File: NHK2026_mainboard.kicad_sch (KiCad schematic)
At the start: 2 parts, among them J1 ABS_Encoder, U1 STM32H753ZITx

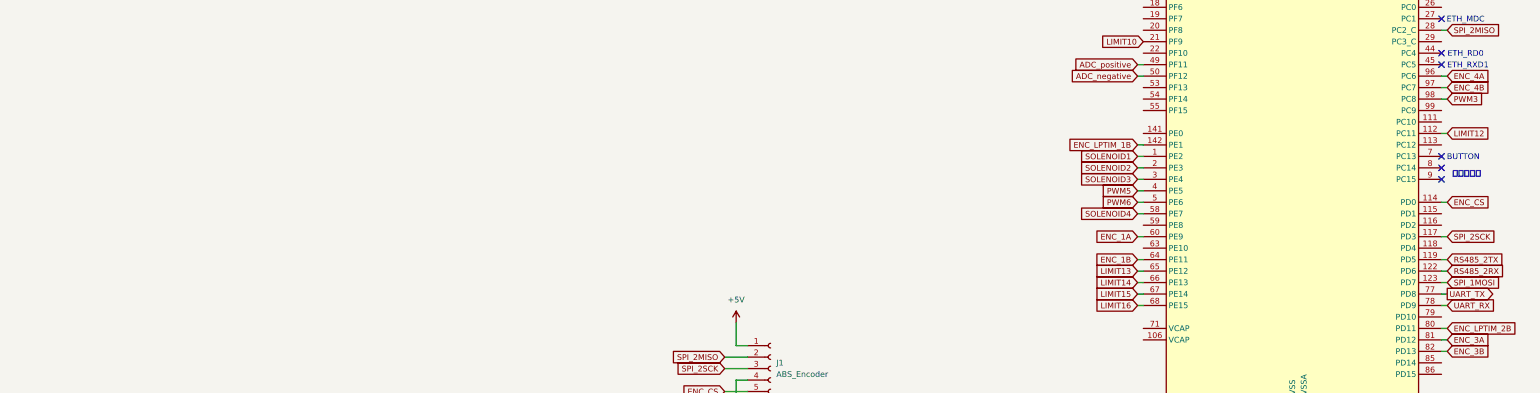
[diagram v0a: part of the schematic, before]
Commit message: 今日はここまで
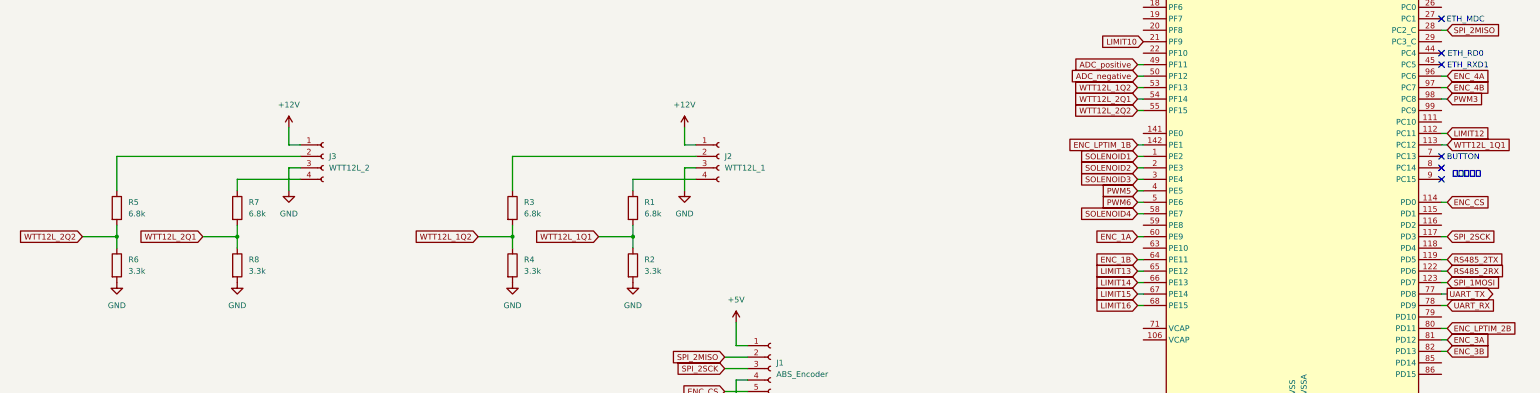
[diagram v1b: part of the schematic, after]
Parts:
- added J2: WTT12L_1, symbol Connector:Conn_01x04_Socket
- added J3: WTT12L_2, symbol Connector:Conn_01x04_Socket
- added R1, R3, R5, R7: 6.8k, symbol Device:R
- added R2, R4, R6, R8: 3.3k, symbol Device:R
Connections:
- net GND: now also J2.3 (Pin_3), J3.3 (Pin_3), R2.2, R4.2, R6.2, R8.2
- net WTT12L_1Q1: now reaches U1.113 (PC12)
- net WTT12L_1Q1: now also R1.2, R2.1
- net WTT12L_1Q2: now reaches U1.53 (PF13)
- net WTT12L_1Q2: now also R3.2, R4.1
- net WTT12L_2Q1: now reaches U1.54 (PF14)
- net WTT12L_2Q1: now also R7.2, R8.1
- net WTT12L_2Q2: now reaches U1.55 (PF15)
- net WTT12L_2Q2: now also R5.2, R6.1
- new net: J2.2 (Pin_2), R3.1
- new net: J3.2 (Pin_2), R5.1
- new net: J3.4 (Pin_4), R7.1
- new net: J2.4 (Pin_4), R1.1
- new net +12V: J2.1 (Pin_1), J3.1 (Pin_1)

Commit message: 恥を捨て豊橋スタイル丸パクリ
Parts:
- removed J2: WTT12L_1, symbol Connector:Conn_01x04_Socket
- removed J3: WTT12L_2, symbol Connector:Conn_01x04_Socket
- removed R1, R3, R5, R7: 6.8k, symbol Device:R
- removed R2, R4, R6, R8: 3.3k, symbol Device:R
- added C?: 0.1u, symbol Device:C
- added C?: 0.1u, Capacitor_SMD:C_0603_1608Metric_Pad1.08x0.95mm_HandSolder, symbol Device:C
- added J?: SPI, symbol Connector:Conn_01x04_Socket
- added J?: ADC, symbol Connector:Conn_01x02_Socket
- added J?: I2C, symbol Connector:Conn_01x03_Socket
- added J?: SOLENOID_1, Connector_JST:JST_XH_S5B-XH-A-1_1x05_P2.50mm_Horizontal, symbol Connector:Conn_01x05_Socket
- added U?: BNO055, MyLib:BNO055, symbol MyLib:BNO055
- added U?: TXRX_pokayoke, Mylib:TXRX_pokayoke, symbol MyLib:TXRX_pokayoke
- renumbered J1 to J?, U1 to U?
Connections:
- net +5V: now also C?.1
- net ADC_negative: now also J?.2 (Pin_2)
- net ADC_positive: now also J?.1 (Pin_1)
- net BNO_RX: now also U?.3 (RX1)
- net BNO_TX: now also U?.1 (TX1)
- net GND: now also C?.2, C?.2, J?.1 (Pin_1), J?.1 (Pin_1), J?.1 (Pin_1), U?.2 (GND), U?.6 (GND)
- net I2C_SCL: now also J?.3 (Pin_3)
- net I2C_SDA: now also J?.2 (Pin_2)
- net SOLENOID1: now also J?.2 (Pin_2)
- net SOLENOID2: now also J?.3 (Pin_3)
- net SOLENOID3: now also J?.4 (Pin_4)
- net SOLENOID4: now also J?.5 (Pin_5)
- net SPI_1MISO: now also J?.3 (Pin_3)
- net SPI_1MOSI: now also J?.2 (Pin_2)
- net SPI_1SCK: now also J?.4 (Pin_4)
- net DIR1: now reaches U?.12 (PF2)
- net DIR2: now reaches U?.13 (PF3)
- net DIR3: now reaches U?.14 (PF4)
- net DIR4: now reaches U?.15 (PF5)
- net WTT12L_3Q1: now reaches U?.63 (PE10)
- net WTT12L_3Q2: now reaches U?.70 (PB11)
- net PWM7: now reaches U?.75 (PB14)
- net PWM8: now reaches U?.76 (PB15)
- new net: U?.3 (SDA), U?.4 (TX2)
- new net: U?.2 (RX2), U?.4 (SCL)
- new net +3V3: C?.1, U?.1 (VIN)
- no-connect marks 17 -> 19
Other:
- added sheet CAN (can.kicad_sch)
- added sheet ENCODER (encoder.kicad_sch)
- added sheet LIMIT_SWITCH (limit_switch.kicad_sch)
- added sheet MOTOR (motor.kicad_sch)
- added sheet REGULATOR (regulator.kicad_sch)
- added sheet RS485 (rs485.kicad_sch)
- added sheet WTT12L (wtt12l.kicad_sch)
- note added: "WTT12L_3QxのCubeMXの更新わすれずに PB14,PB15のサーボ用PWMわすれずに PF2,PF3,PF4,PF5のDIRわすれずに ENC_3Bの確認"
- note removed: "LD3"
- moved on the sheet: J?, U?

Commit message: 回路図だいたい完成
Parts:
- removed U?: STM32H753ZITx, MyLib:MODULE_NUCLEO-H753ZI, symbol MCU_ST_STM32H7:STM32H753ZITx
- added J43: PicoScan, symbol Connector:Conn_01x02_Socket
- added R50: 10k, symbol Device:R
- added SW1: SW_Push, symbol Switch:SW_Push
- added U14: NUCLEO-H753ZI, NUCLEO-H753ZI:MODULE_NUCLEO-H753ZI, symbol MyLib:NUCLEO-H753ZI
- gave numbers to parts that had none: 9
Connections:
- net +3V3: now also R50.1, U14.CN11_16 (3V3)
- net +5V: now also U14.CN11_6 (5V_EXT)
- net ADC_negative: now also U14.CN12_59 (PF12)
- net ADC_positive: now also U14.CN12_62 (PF11)
- net BNO_RX: now also U14.CN11_63 (PG9)
- net BNO_TX: now also U14.CN12_61 (PG14)
- net DIR1: now also U14.CN12_58 (PF3)
- net DIR2: now also U14.CN12_38 (PF4)
- net DIR3: now also U14.CN12_36 (PF5)
- net DIR4: now also U14.CN12_42 (PF10)
- net ENC_1A: now also U14.CN12_52 (PE9)
- net ENC_1B: now also U14.CN12_56 (PE11)
- net ENC_2A: now also U14.CN11_28 (PA0)
- net ENC_2B: now also U14.CN12_31 (PB3)
- net ENC_3A: now also U14.CN12_43 (PD12)
- net ENC_3B: now also U14.CN12_41 (PD13)
- net ENC_4A: now also U14.CN12_4 (PC6)
- net ENC_4B: now also U14.CN12_19 (PC7)
- net ENC_CS: now also U14.CN11_57 (PD0)
- net ENC_LPTIM_1A: now also U14.CN11_65 (PG12)
- net ENC_LPTIM_1B: now also U14.CN11_61 (PE1)
- net ENC_LPTIM_2A: now also U14.CN12_25 (PB10)
- net ENC_LPTIM_2B: now also U14.CN12_45 (PD11)
- net FDCAN_1RX: now also U14.CN12_14 (PA11)
- net FDCAN_1TX: now also U14.CN12_12 (PA12)
- net FDCAN_2RX: now also U14.CN12_16 (PB12)
- net FDCAN_2TX: now also U14.CN12_17 (PB6)
- net GND: now also J43.2 (Pin_2), SW1.2, U14.CN11_19 (GND_CN11), U14.CN11_20 (GND_CN11), U14.CN11_22 (GND_CN11), U14.CN11_49 (GND_CN11), U14.CN11_60 (GND_CN11), U14.CN11_71 (GND_CN11), U14.CN11_72 (GND_CN11), U14.CN11_8 (GND_CN11), U14.CN12_20 (GND_CN12), U14.CN12_32 (AGND_CN12), U14.CN12_39 (GND_CN12), U14.CN12_54 (GND_CN12), U14.CN12_63 (GND_CN12), U14.CN12_71 (GND_CN12), U14.CN12_72 (GND_CN12), U14.CN12_9 (GND_CN12)
- net I2C_SCL: now also U14.CN11_51 (PF1)
- net I2C_SDA: now also U14.CN11_53 (PF0)
- net LIMIT1: now also U14.CN11_59 (PG0)
- net LIMIT10: now also U14.CN11_56 (PF9)
- net LIMIT11: now also U14.CN11_66 (PG10)
- net LIMIT12: now also U14.CN11_2 (PC11)
- net LIMIT13: now also U14.CN12_49 (PE12)
- net LIMIT14: now also U14.CN12_55 (PE13)
- net LIMIT15: now also U14.CN12_51 (PE14)
- net LIMIT16: now also U14.CN12_53 (PE15)
- net LIMIT2: now also U14.CN11_58 (PG1)
- net LIMIT3: now also U14.CN11_42 (PG2)
- net LIMIT4: now also U14.CN11_44 (PG3)
- net LIMIT5: now also U14.CN12_69 (PG4)
- net LIMIT6: now also U14.CN12_68 (PG5)
- net LIMIT7: now also U14.CN12_70 (PG6)
- net LIMIT8: now also U14.CN12_67 (PG7)
- net LIMIT9: now also U14.CN12_66 (PG8)
- net PWM1: now also U14.CN12_13 (PA6)
- net PWM2: now also U14.CN12_29 (PB5)
- net PWM3: now also U14.CN12_2 (PC8)
- net PWM4: now also U14.CN12_24 (PB1)
- net PWM5: now also U14.CN11_50 (PE5)
- net PWM6: now also U14.CN11_62 (PE6)
- net PWM7: now also U14.CN12_28 (PB14)
- net PWM8: now also U14.CN12_26 (PB15)
- net RS485_1RX: now also U14.CN12_33 (PA10)
- net RS485_1TX: now also U14.CN12_21 (PA9)
- net RS485_2RX: now also U14.CN11_43 (PD6)
- net RS485_2TX: now also U14.CN11_41 (PD5)
- net SOLENOID1: now also U14.CN11_32 (PA4)
- net SOLENOID2: now also U14.CN11_13 (PA13)
- net SOLENOID3: now also U14.CN11_15 (PA14)
- net SOLENOID4: now also U14.CN11_17 (PA15)
- net SPI_1MISO: now also U14.CN12_27 (PB4)
- net SPI_1MOSI: now also U14.CN11_45 (PD7)
- net SPI_1SCK: now also U14.CN12_11 (PA5)
- net SPI_2MISO: now also U14.CN11_35 (PC2)
- net SPI_2SCK: now also U14.CN11_40 (PD3)
- net WTT12L_1Q1: now also U14.CN11_3 (PC12)
- net WTT12L_1Q2: now also U14.CN12_57 (PF13)
- net WTT12L_2Q1: now also U14.CN12_50 (PF14)
- net WTT12L_2Q2: now also U14.CN12_60 (PF15)
- net WTT12L_3Q1: now also U14.CN12_47 (PE10)
- net WTT12L_3Q2: now also U14.CN12_18 (PB11)
- new net: R50.2, SW1.1, U14.CN11_14 (NRST)
- new net: U14.CN11_10 (NC), U14.CN11_26 (NC), U14.CN11_67 (NC)
- new net +12V: J43.1 (Pin_1)
- no-connect marks 19 -> 24
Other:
- note added: "ETH_RXD0"
- note added: "PicoScanの電源"
- note added: "UART_RX"
- note added: "UART_TX"
- note added: "使用可能"
- note removed: "ETH_RD0"
- note removed: "ETH_TXD0"
- note removed: "WTT12L_3QxのCubeMXの更新わすれずに PB14,PB15のサーボ用PWMわすれずに PF2,PF3,PF4,PF5のDIRわすれずに ENC_3Bの確認"
- moved on the sheet: C13, J13, J14, J15, J16, J17
